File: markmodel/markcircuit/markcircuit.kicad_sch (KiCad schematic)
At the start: 19 parts, among them M1 Motor_Servo, M2 Motor_Servo, SW2 SW_DPST_x2, SW3 SW_Push, U1 ATmega328-P

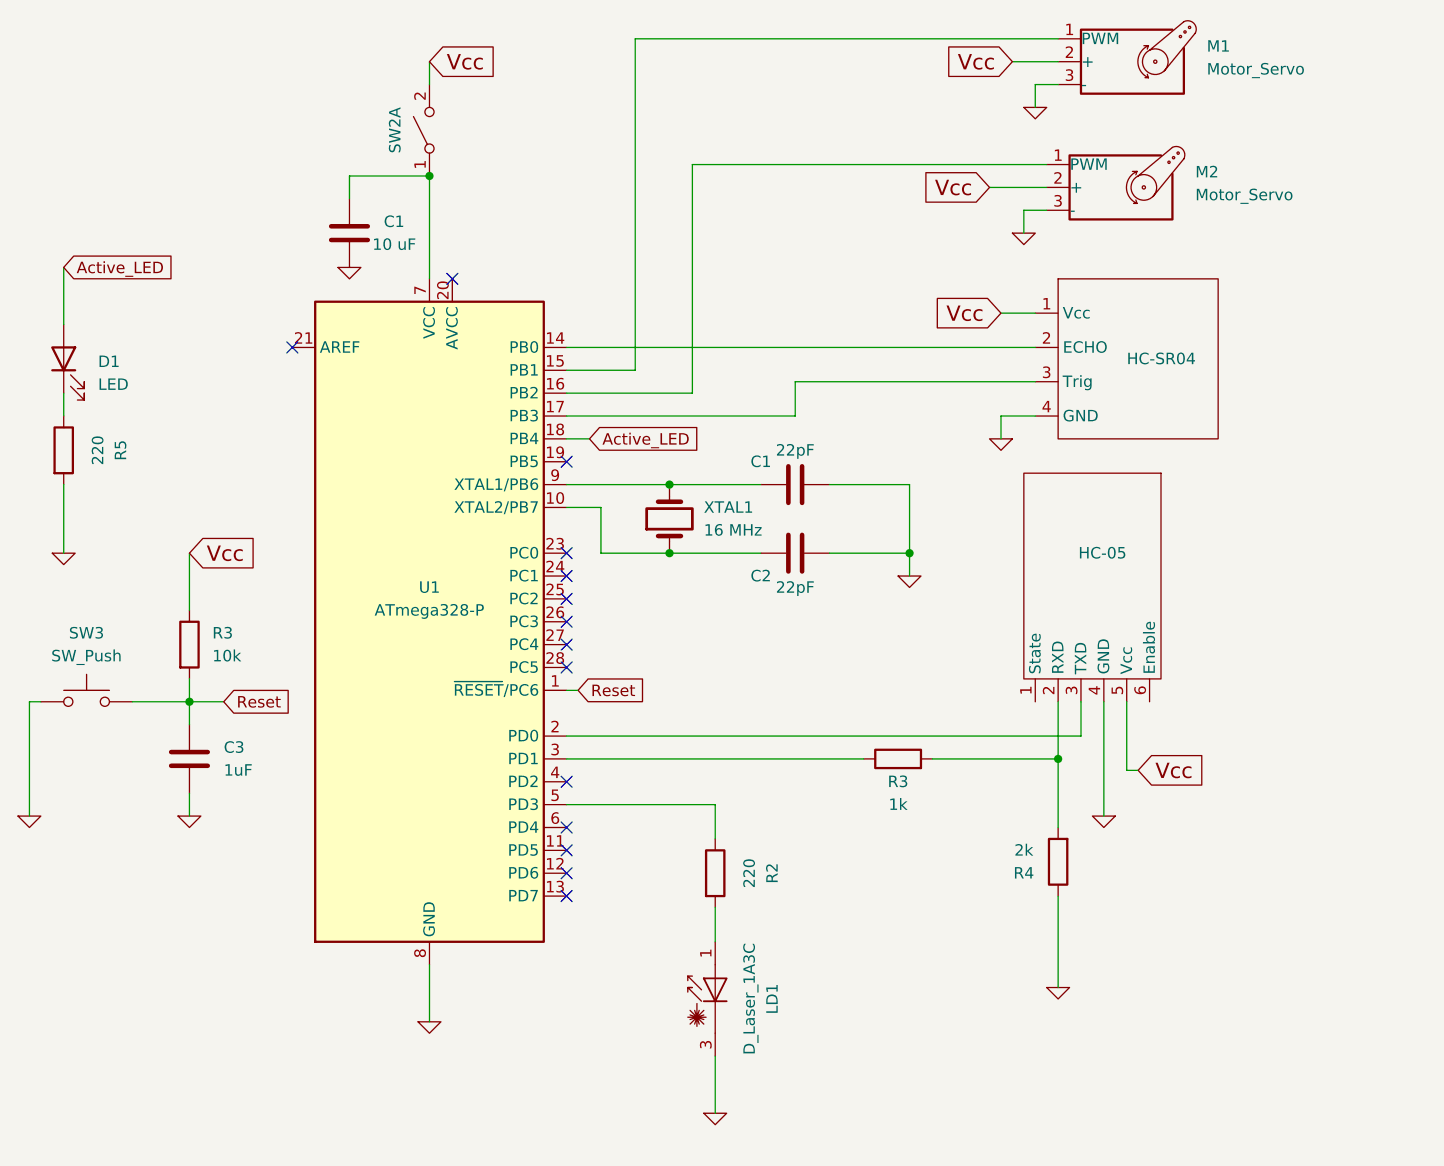
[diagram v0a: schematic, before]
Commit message: finished.
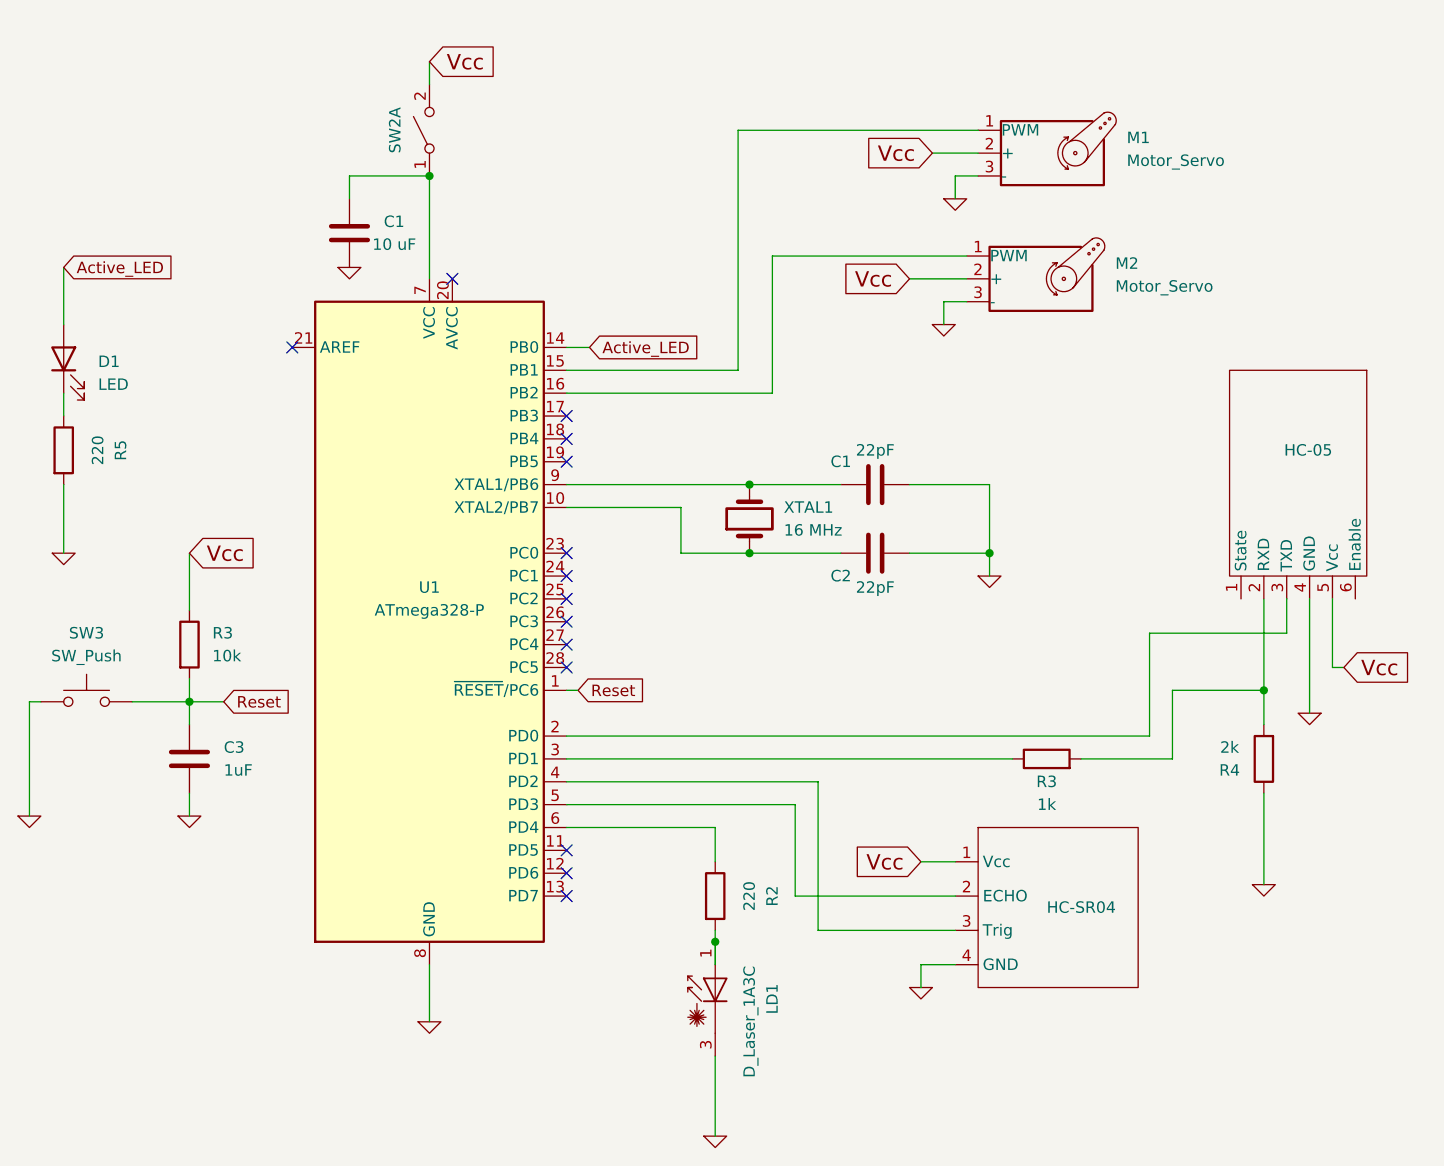
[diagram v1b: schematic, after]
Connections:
- net Active_LED: now also U1.14 (PB0); no longer U1.18 (PB4)
- net at R2.1: now also U1.6 (PD4); no longer U1.5 (PD3)
- net at HC-SR04.2 (ECHO): now also U1.5 (PD3); no longer U1.14 (PB0)
- net at HC-SR04.3 (Trig): now also U1.4 (PD2); no longer U1.17 (PB3)
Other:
- moved on the sheet: C1, C2, HC-05, HC-SR04, M1, M2, R2, R3, R4, XTAL1
